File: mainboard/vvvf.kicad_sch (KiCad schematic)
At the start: 92 parts, among them J1 Connector to external IGBT Mo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, J10 Conn_01x05_Pin, J6 Screw_Terminal_01x02, J9 Screw_Terminal_01x02, Q1 Q_NIGBT_GCE, Q2 Q_NIGBT_GCE, SW1 SW_Push, U1 TLP152, U11 LM7805_TO220, U2 TLP152, U3 UCC21520ADW, U4 TLP152, U5 MCP3421A0T-ECH, U6 UCC21520ADW, U7 UCC21520ADW, U8 ISO1540

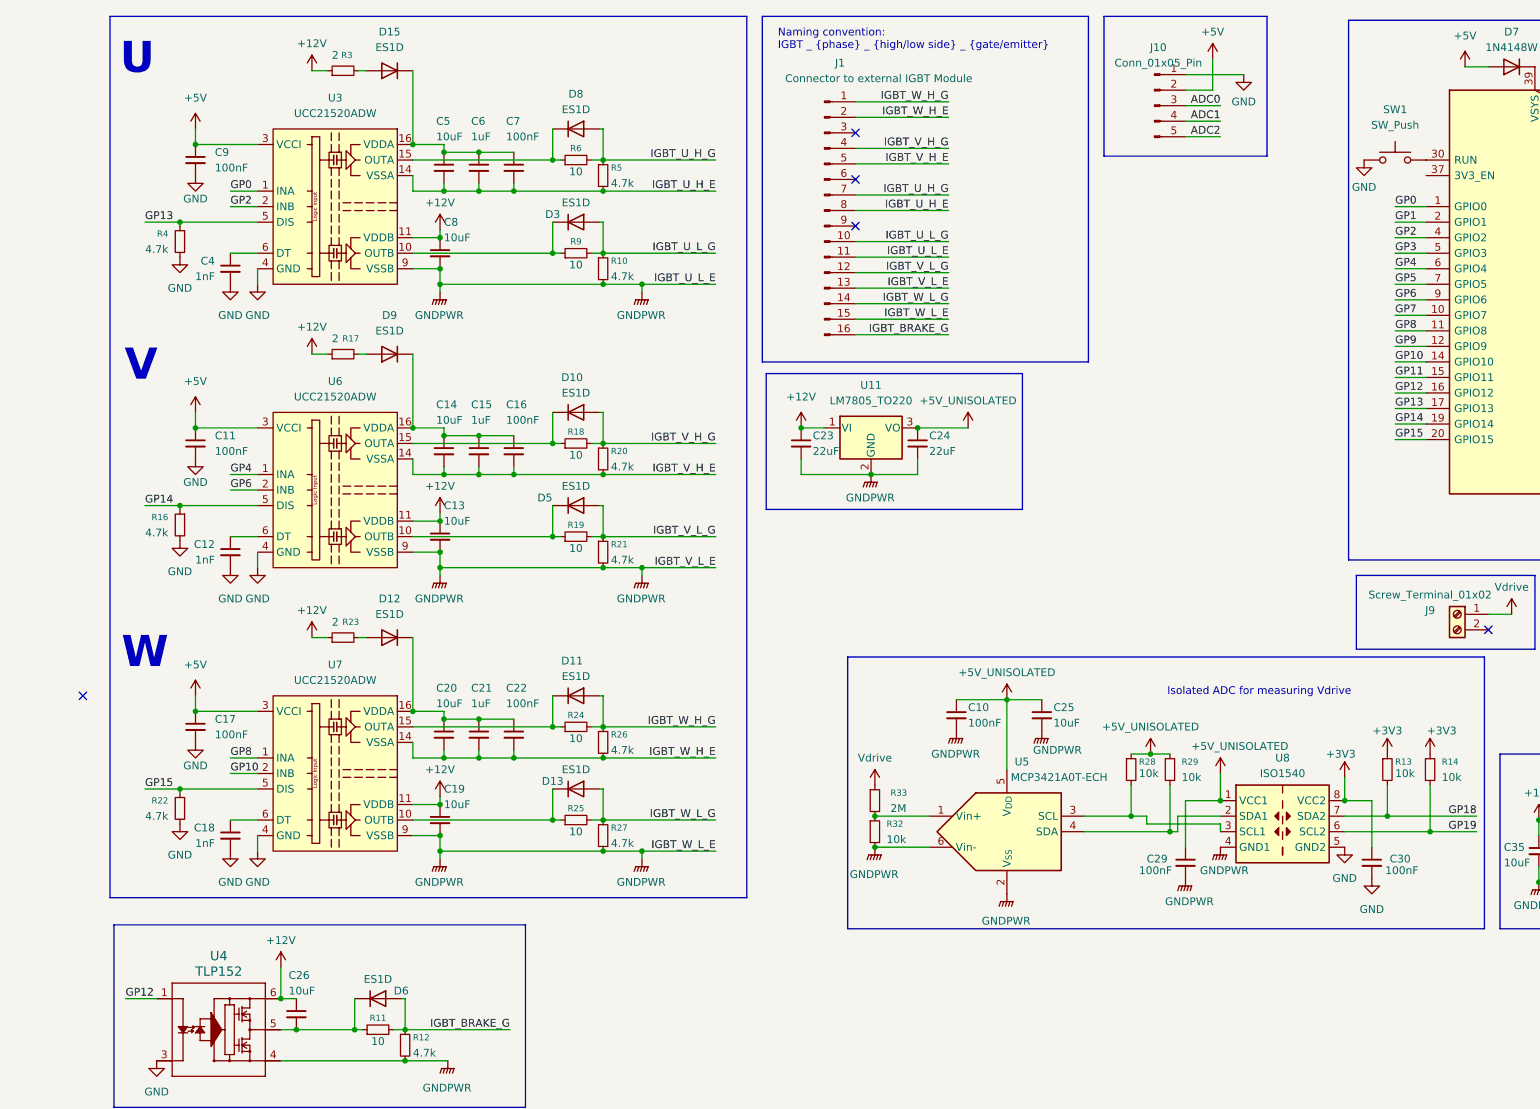
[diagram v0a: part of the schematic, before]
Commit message: order for mainboard v1.0
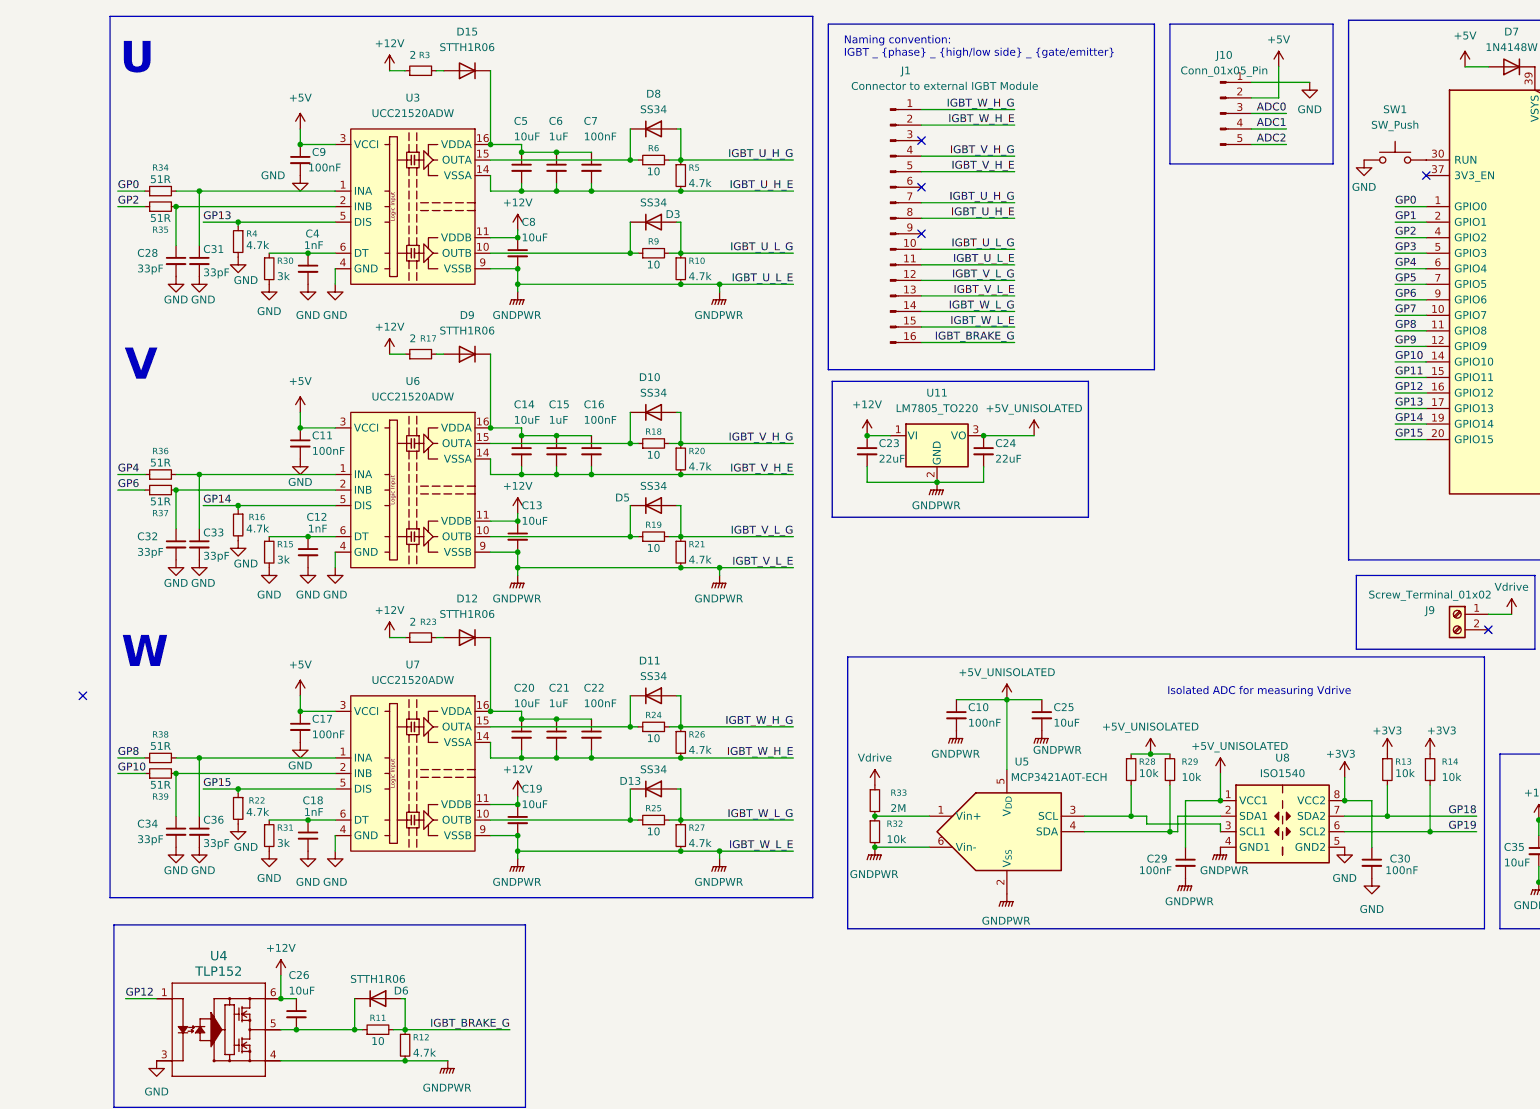
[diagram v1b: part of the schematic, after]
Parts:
- added C28, C31, C32, C33, C34, C36: 33pF, Capacitor_SMD:C_0603_1608Metric_Pad1.08x0.95mm_HandSolder, symbol Device:C_Small
- added R15, R30, R31: 3k, Capacitor_SMD:C_0603_1608Metric_Pad1.08x0.95mm_HandSolder, symbol Device:R_Small
- added R34, R35, R36, R37, R38, R39: 51R, Resistor_SMD:R_0603_1608Metric_Pad0.98x0.95mm_HandSolder, symbol Device:R_Small
- A1, J1, J10, J6, J9: LCSC Part (none) -> N/A
- C10, C11, C16, C17, C22, C29, C30, C7, C9: LCSC Part (none) -> C14663
- C12, C18, C4: LCSC Part (none) -> C1588
- C13, C14, C19, C20, C25, C26, C27, C35, C5, C8: LCSC Part (none) -> C194427
- C15, C21, C6: LCSC Part (none) -> C15849
- C23, C24: LCSC Part (none) -> C29519229
- D10, D11, D13, D3, D5, D8: value ES1D -> SS34; footprint Diode_SMD:D_SMA_Handsoldering -> Diode_SMD:D_SMA; LCSC Part (none) -> C8678
- D12, D15, D6, D9: value ES1D -> STTH1R06; footprint Diode_SMD:D_SMA_Handsoldering -> Diode_THT:D_DO-41_SOD81_P7.62mm_Horizontal; LCSC Part (none) -> C2971307
- D7: LCSC Part (none) -> C241939
- R10, R12, R16, R20, R21, R22, R26, R27, R4, R5: LCSC Part (none) -> C99782
- R11, R18, R19, R24, R25, R6, R9: LCSC Part (none) -> C510088
- R13, R14, R28, R29: LCSC Part (none) -> C98220
- R17, R23, R3: footprint Resistor_SMD:R_0603_1608Metric_Pad0.98x0.95mm_HandSolder -> Resistor_SMD:R_1210_3225Metric_Pad1.30x2.65mm_HandSolder; LCSC Part (none) -> C620674
- SW1: LCSC Part (none) -> C455282
- U11: LCSC Part (none) -> C7432180
- U3, U6, U7: LCSC Part C2863027 -> C601651
- U4: LCSC Part (none) -> C150122
- U5: LCSC Part (none) -> C29454
- U8: LCSC Part (none) -> C179739
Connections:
- net GND: now also C28.2, C31.2, C32.2, C33.2, C34.2, C36.2, R15.2, R30.2, R31.2
- net GP0: now also R34.1; no longer U3.1 (INA)
- net GP10: now also R39.1; no longer U7.2 (INB)
- net GP2: now also R35.1; no longer U3.2 (INB)
- net GP4: now also R36.1; no longer U6.1 (INA)
- net GP6: now also R37.1; no longer U6.2 (INB)
- net GP8: now also R38.1; no longer U7.1 (INA)
- net at C12.1, U6.6 (DT): now also R15.1
- net at C18.1, U7.6 (DT): now also R31.1
- net at C4.1, U3.6 (DT): now also R30.1
- new net: C36.1, R38.2, U7.1 (INA)
- new net: C33.1, R36.2, U6.1 (INA)
- new net: C28.1, R35.2, U3.2 (INB)
- new net: C32.1, R37.2, U6.2 (INB)
- new net: C34.1, R39.2, U7.2 (INB)
- new net: C31.1, R34.2, U3.1 (INA)
- no-connect marks 8 -> 9
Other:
- moved on the sheet: C11, C12, C13, C14, C15, C16, C17, C18, C19, C20, C21, C22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
